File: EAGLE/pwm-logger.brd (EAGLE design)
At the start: 41.6 x 33 mm, 29 parts, among them U1 24LC256, U2 3.3V/150mA

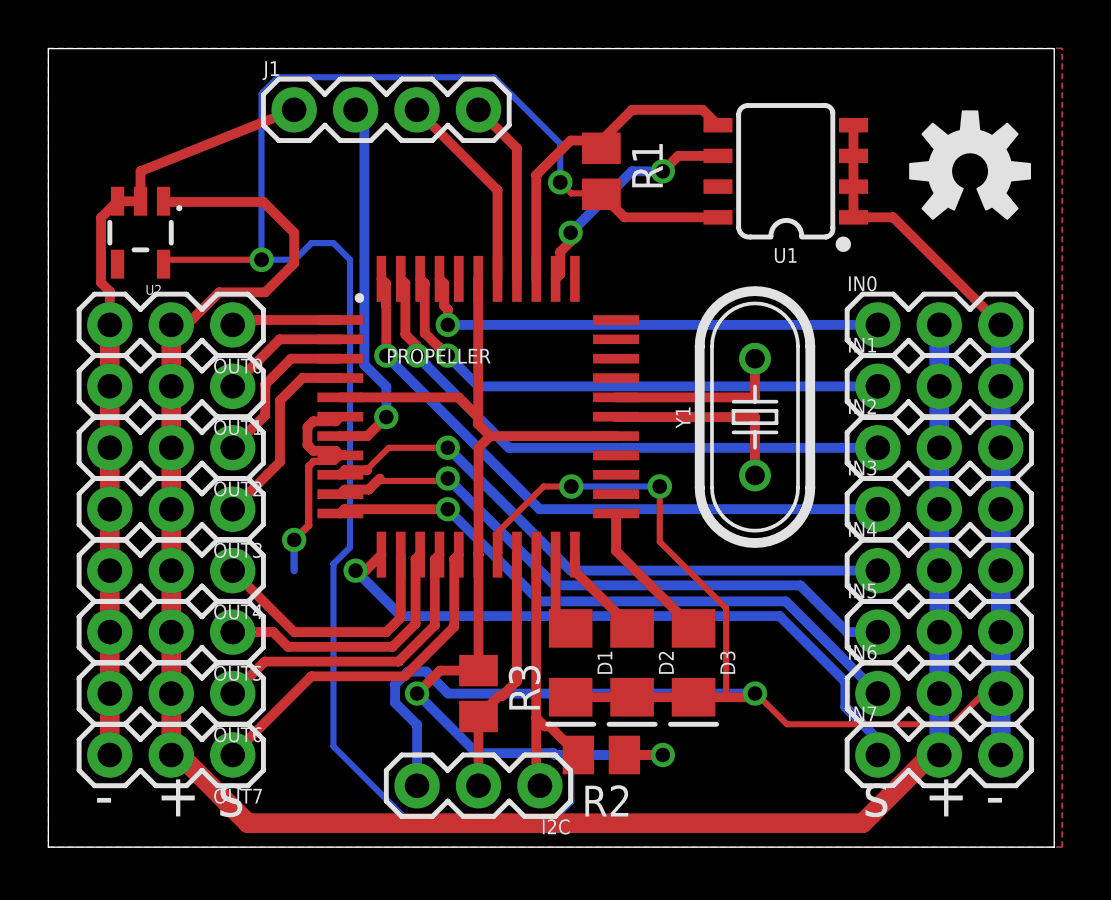
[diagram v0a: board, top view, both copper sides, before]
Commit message: Updated schematics
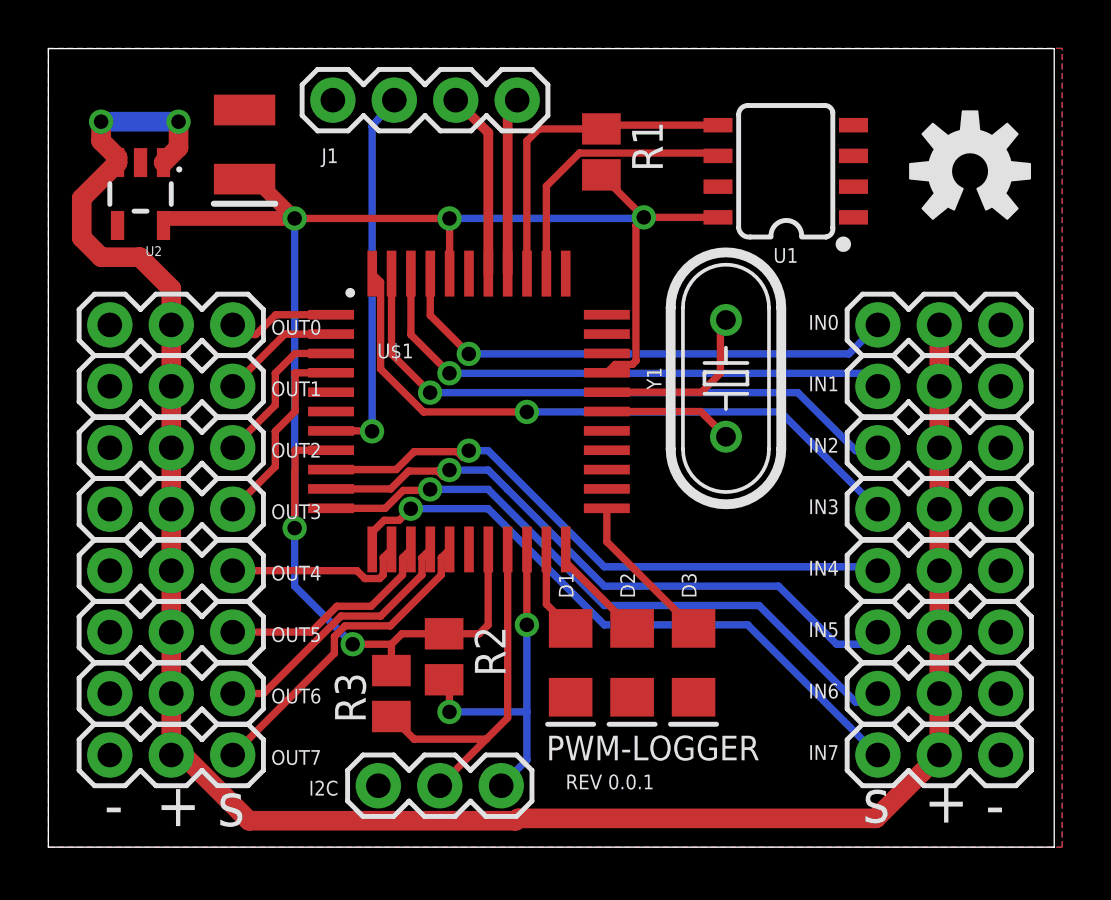
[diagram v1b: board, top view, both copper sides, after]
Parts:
- removed PROPELLER: PROPELLER-44Q, parallax:Q44
- added C1: 330UF-POLAR, SparkFun-Capacitors:1311
- added U$1: PROPELLER-44Q, parallax:Q44
- Y1: value (none) -> 5 MHz
- moved R2 7.66 mm to (49.4, 37.1), turned to 270 degrees
- moved R3 3.60 mm to (47.2, 35.6)
- moved Y1 2.00 mm to (61.0, 48.6)
- moved J1 1.65 mm to (44.8, 60.1)
- moved I2C 1.60 mm to (51.7, 31.8)
- moved U2 1.60 mm to (36.8, 56.2)
- moved R1 0.80 mm to (55.9, 58.0)
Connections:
- net IN0: now also U$1.41; no longer PROPELLER.41
- net IN1: now also U$1.42; no longer PROPELLER.42
- net IN2: now also U$1.43; no longer PROPELLER.43
- net IN3: now also U$1.44; no longer PROPELLER.44
- net IN4: now also U$1.9; no longer PROPELLER.9
- net IN5: now also U$1.10; no longer PROPELLER.10
- net IN6: now also U$1.11; no longer PROPELLER.11
- net IN7: now also U$1.12; no longer PROPELLER.12
- net N$1: now also U$1.28; no longer PROPELLER.28
- net N$2: now also U$1.29; no longer PROPELLER.29
- net N$3: now also U$1.23; no longer PROPELLER.23
- net N$4: now also U$1.22; no longer PROPELLER.22
- net N$5: now also U$1.38; no longer PROPELLER.38
- net N$6: now also U$1.21; no longer PROPELLER.21
- net N$8: now also U$1.37; no longer PROPELLER.37
- net OUT0: now also U$1.1; no longer PROPELLER.1
- net OUT1: now also U$1.2; no longer PROPELLER.2
- net OUT2: now also U$1.3; no longer PROPELLER.3
- net OUT3: now also U$1.4; no longer PROPELLER.4
- net OUT4: now also U$1.13; no longer PROPELLER.13
- net OUT5: now also U$1.14; no longer PROPELLER.14
- net OUT6: now also U$1.15; no longer PROPELLER.15
- net OUT7: now also U$1.16; no longer PROPELLER.16
- net POWER_IN: now also U2.3
- net RES: now also U$1.7; no longer PROPELLER.7
- net SCL: now also U$1.20; no longer PROPELLER.20
- net SCL_EEP: now also U$1.35; no longer PROPELLER.35
- net SDA: now also U$1.19; no longer PROPELLER.19
- net SDA_EEP: now also U$1.36; no longer PROPELLER.36
- net VDD: now also C1.+, U$1.18, U$1.30, U$1.40, U$1.8; no longer PROPELLER.17, PROPELLER.27, PROPELLER.39, PROPELLER.5
- net VSS: now also C1.-, U$1.17, U$1.27, U$1.39, U$1.5, U$1.6, U2.4; no longer PROPELLER.18, PROPELLER.30, PROPELLER.40, PROPELLER.6, PROPELLER.8, U2.3
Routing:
- net VSS: track 129.3 -> 0.00 mm, vias 4 -> 0
- net VDD: track 115.0 -> 71.5 mm, vias 4 -> 5
- net SDA: track 10.3 -> 15.2 mm
- net POWER_IN: track 83.0 -> 86.6 mm, vias 0 -> 2
- net OUT4: track 10.9 -> 7.62 mm
- net SCL: track 12.0 -> 14.8 mm, vias 0 -> 2
- net N$1: track 8.17 -> 5.35 mm
- net OUT5: track 11.1 -> 9.20 mm
- net SCL_EEP: track 9.57 -> 11.3 mm, vias 2 -> 0
- net IN0: track 19.8 -> 21.4 mm
- net OUT6: track 12.5 -> 11.1 mm
- net IN6: track 25.5 -> 26.7 mm
- net IN5: track 25.2 -> 26.3 mm
- net OUT7: track 14.4 -> 13.3 mm
- net IN2: track 24.1 -> 25.1 mm
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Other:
- board text added: "PWM-LOGGER"
- board text added: "REV 0.0.1"
